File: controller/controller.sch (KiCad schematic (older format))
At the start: 33 parts, among them J1 Arduino_Nano_Header, P1 CONN_01X03, P2 CONN_01X03, P3 CONN_01X07, P4 CONN_01X02, P5 CONN_01X10, P6 CONN_01X08, SW1 DIPS_10, U1 MAX5024, U3 IL610, U4 MAX3040, U5 74LS165, U6 74LS165

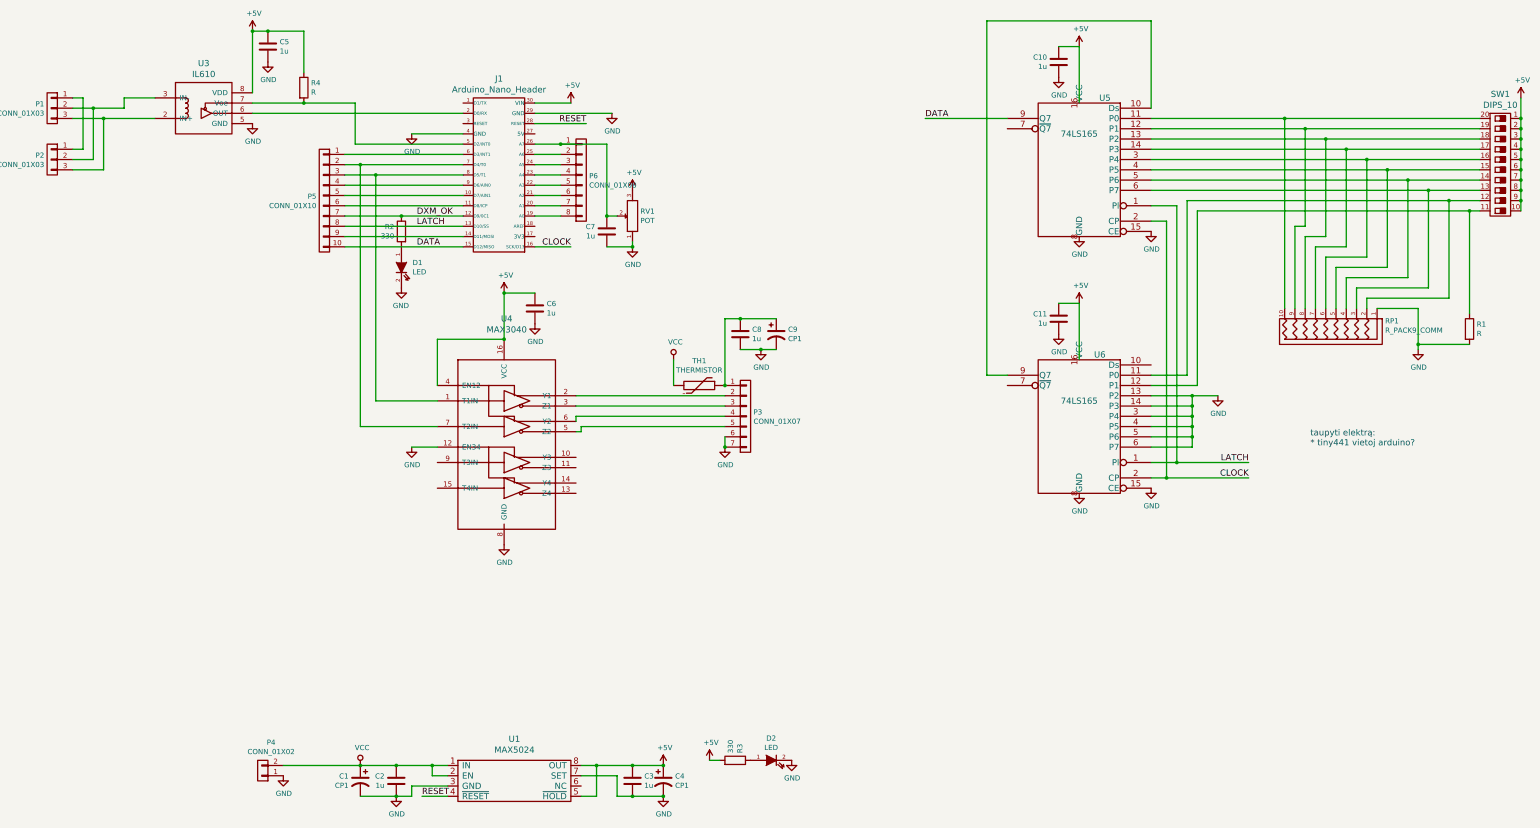
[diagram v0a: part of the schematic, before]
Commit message: Forgotten commit at the end of project
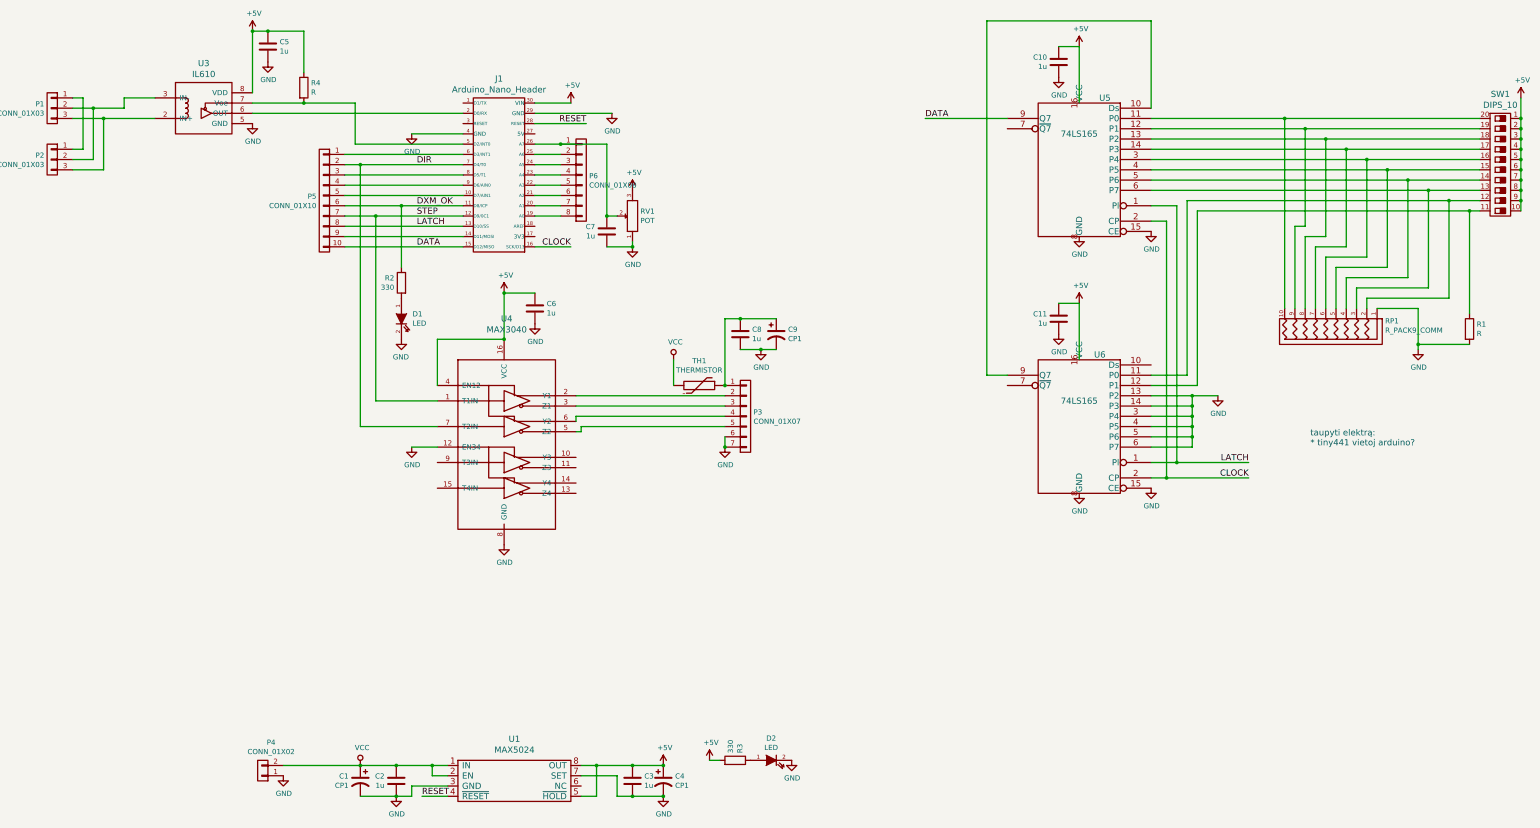
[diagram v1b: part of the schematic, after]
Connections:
- net DXM_OK: now also J1.11 (D8/ICP), P5.6 (P6); no longer J1.12 (D9/0C1), P5.7 (P7)
- net at J1.8 (D5/T1), P5.3 (P3): no longer U4.1 (T1IN)
- net DIR: now reaches J1.7 (D4/T0), P5.2 (P2), U4.7 (T2IN)
- new net STEP: J1.12 (D9/0C1), P5.7 (P7), U4.1 (T1IN)
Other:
- moved on the sheet: D1, R2
